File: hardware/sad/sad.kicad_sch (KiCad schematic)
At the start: 37 parts, among them IC1 LP5012RUKR, J1 USB_C_Receptacle_USB2.0_16P, U1 ATtiny1616-M, U2 MCP73831-2-OT

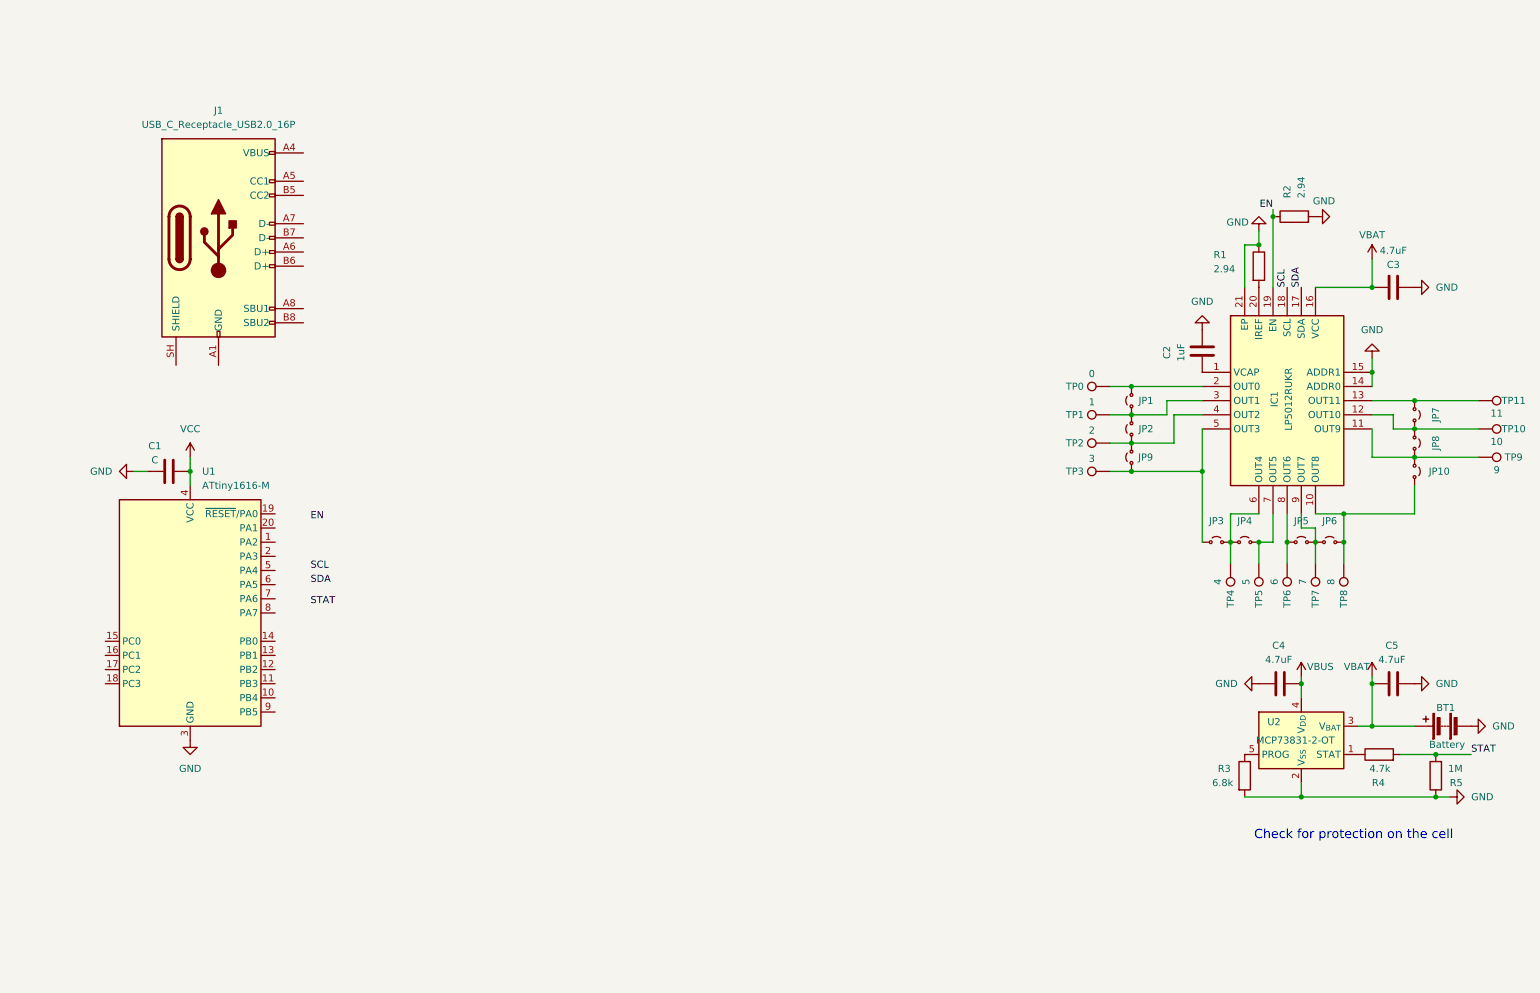
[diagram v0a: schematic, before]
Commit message: init sch finished
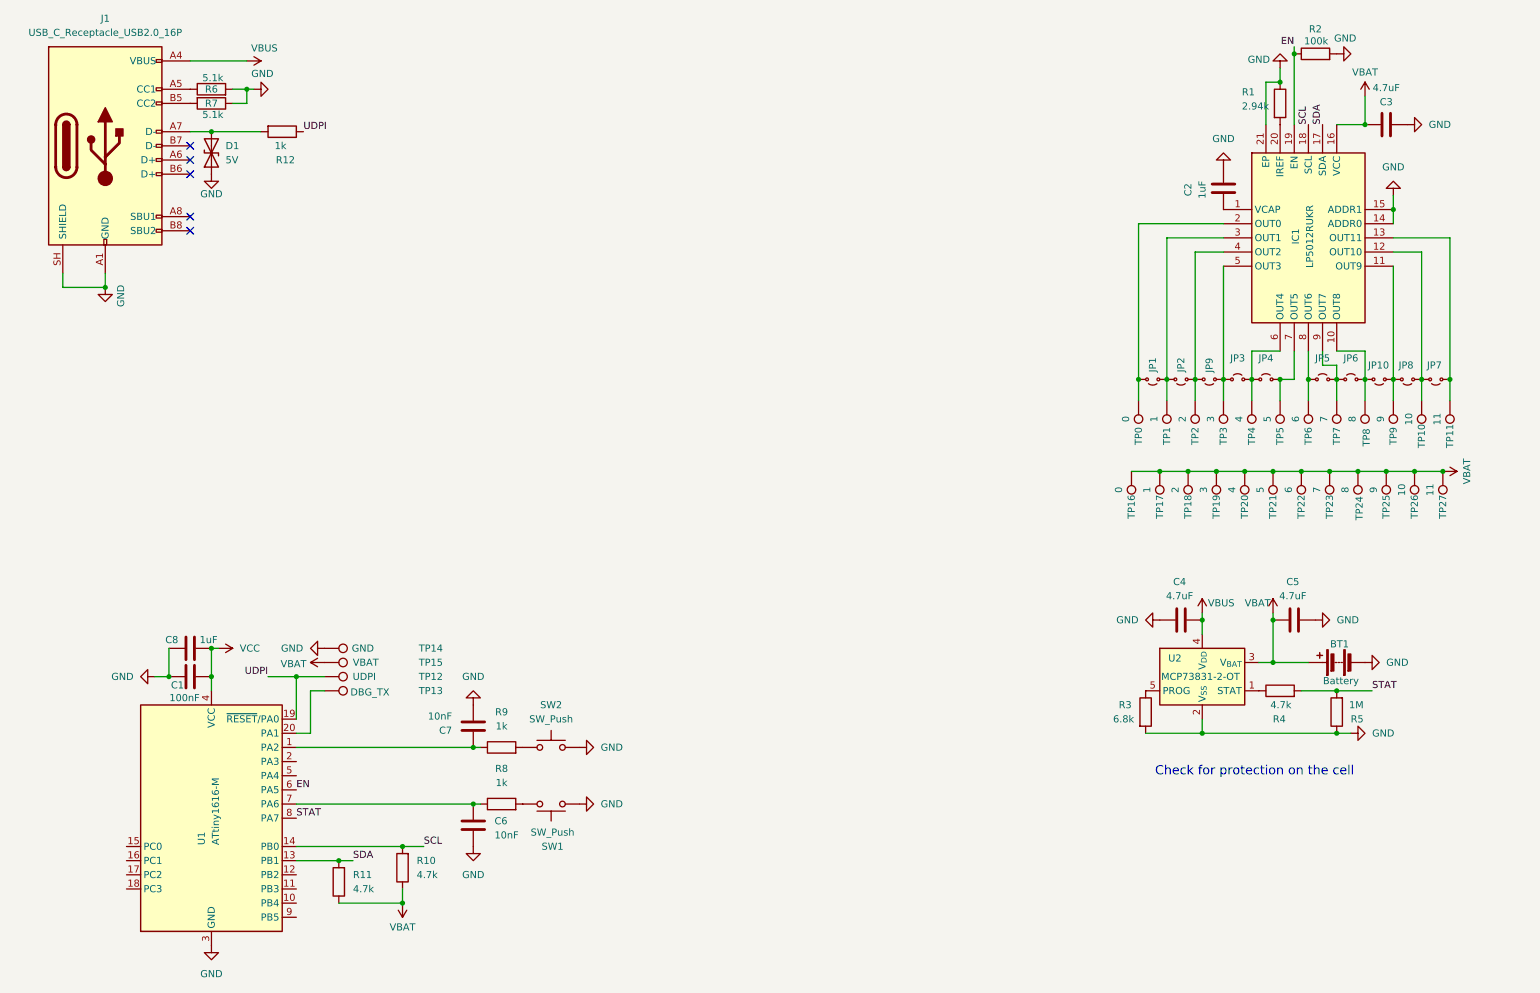
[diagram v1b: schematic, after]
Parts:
- added C6, C7: 10nF, Package_TO_SOT_SMD:SOT-23-5, symbol Device:C
- added C8: 1uF, Package_SO:SOIC-8_3.9x4.9mm_P1.27mm, symbol Device:C
- added D1: 5V, Package_DFN_QFN:QFN-16-1EP_4x4mm_P0.65mm_EP2.1x2.1mm_ThermalVias, symbol Device:D_TVS
- added R10, R11: 4.7k, Package_TO_SOT_SMD:SOT-23-5, symbol Device:R
- added R12, R8, R9: 1k, Package_TO_SOT_SMD:SOT-23-5, symbol Device:R
- added R6, R7: 5.1k, Package_TO_SOT_SMD:SOT-23-5, symbol Device:R
- added SW1, SW2: SW_Push, Button_Switch_SMD:Nidec_Copal_CAS-120A, symbol Switch:SW_Push
- added TP12: UDPI, Relay_THT:Relay_DPDT_Schrack-RT2-FormC_RM5mm, symbol Connector:TestPoint
- added TP13: DBG_TX, Relay_THT:Relay_DPDT_Schrack-RT2-FormC_RM5mm, symbol Connector:TestPoint
- added TP14: GND, Relay_THT:Relay_DPDT_Schrack-RT2-FormC_RM5mm, symbol Connector:TestPoint
- added TP15: VBAT, Relay_THT:Relay_DPDT_Schrack-RT2-FormC_RM5mm, symbol Connector:TestPoint
- added TP16: 0, Relay_THT:Relay_DPDT_Schrack-RT2-FormC_RM5mm, symbol Connector:TestPoint
- added TP17: 1, Relay_THT:Relay_DPDT_Schrack-RT2-FormC_RM5mm, symbol Connector:TestPoint
- added TP18: 2, Relay_THT:Relay_DPDT_Schrack-RT2-FormC_RM5mm, symbol Connector:TestPoint
- added TP19: 3, Relay_THT:Relay_DPDT_Schrack-RT2-FormC_RM5mm, symbol Connector:TestPoint
- added TP20: 4, Relay_THT:Relay_DPDT_Schrack-RT2-FormC_RM5mm, symbol Connector:TestPoint
- added TP21: 5, Relay_THT:Relay_DPDT_Schrack-RT2-FormC_RM5mm, symbol Connector:TestPoint
- added TP22: 6, Relay_THT:Relay_DPDT_Schrack-RT2-FormC_RM5mm, symbol Connector:TestPoint
- added TP23: 7, Relay_THT:Relay_DPDT_Schrack-RT2-FormC_RM5mm, symbol Connector:TestPoint
- added TP24: 8, Relay_THT:Relay_DPDT_Schrack-RT2-FormC_RM5mm, symbol Connector:TestPoint
- added TP25: 9, Relay_THT:Relay_DPDT_Schrack-RT2-FormC_RM5mm, symbol Connector:TestPoint
- added TP26: 10, Relay_THT:Relay_DPDT_Schrack-RT2-FormC_RM5mm, symbol Connector:TestPoint
- added TP27: 11, Relay_THT:Relay_DPDT_Schrack-RT2-FormC_RM5mm, symbol Connector:TestPoint
- C1: value C -> 100nF
- R1: value 2.94 -> 2.94k
- R2: value 2.94 -> 100k
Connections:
- net EN: now also U1.6 (PA5)
- net GND: now also J1.A1 (GND), J1.A12 (GND), J1.B1 (GND), J1.B12 (GND), J1.SH (SHIELD), C6.2, C7.2, C8.2, D1.1 (A1), R6.2, R7.1, SW1.1, SW2.2, TP14.1
- net SCL: now also U1.14 (PB0), R10.2
- net SDA: now also U1.13 (PB1), R11.2
- net STAT: now also U1.8 (PA7)
- net VBAT: now also R10.1, R11.1, TP15.1, TP16.1, TP17.1, TP18.1, TP19.1, TP20.1, TP21.1, TP22.1, TP23.1, TP24.1, TP25.1, TP26.1, TP27.1
- net VBUS: now also J1.A4 (VBUS), J1.A9 (VBUS), J1.B4 (VBUS), J1.B9 (VBUS)
- net VCC: now also C8.1
- net at U1.1 (PA2): now also C7.1, R9.1
- net UDPI: now reaches U1.19 (~{RESET}/PA0)
- net UDPI: now also R12.1, TP12.1
- net at U1.20 (PA1): now also TP13.1
- net at U1.7 (PA6): now also C6.1, R8.1
- net at J1.A5 (CC1): now also R6.1
- net at J1.A7 (D-): now also D1.2 (A2), R12.2
- net at J1.B5 (CC2): now also R7.2
- new net: R9.2, SW2.1
- new net: R8.2, SW1.2
- no-connect marks 0 -> 5
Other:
- moved on the sheet: BT1, C1, C2, C3, C4, C5, IC1, J1, JP1, JP10, JP2, JP3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

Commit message: rearranged
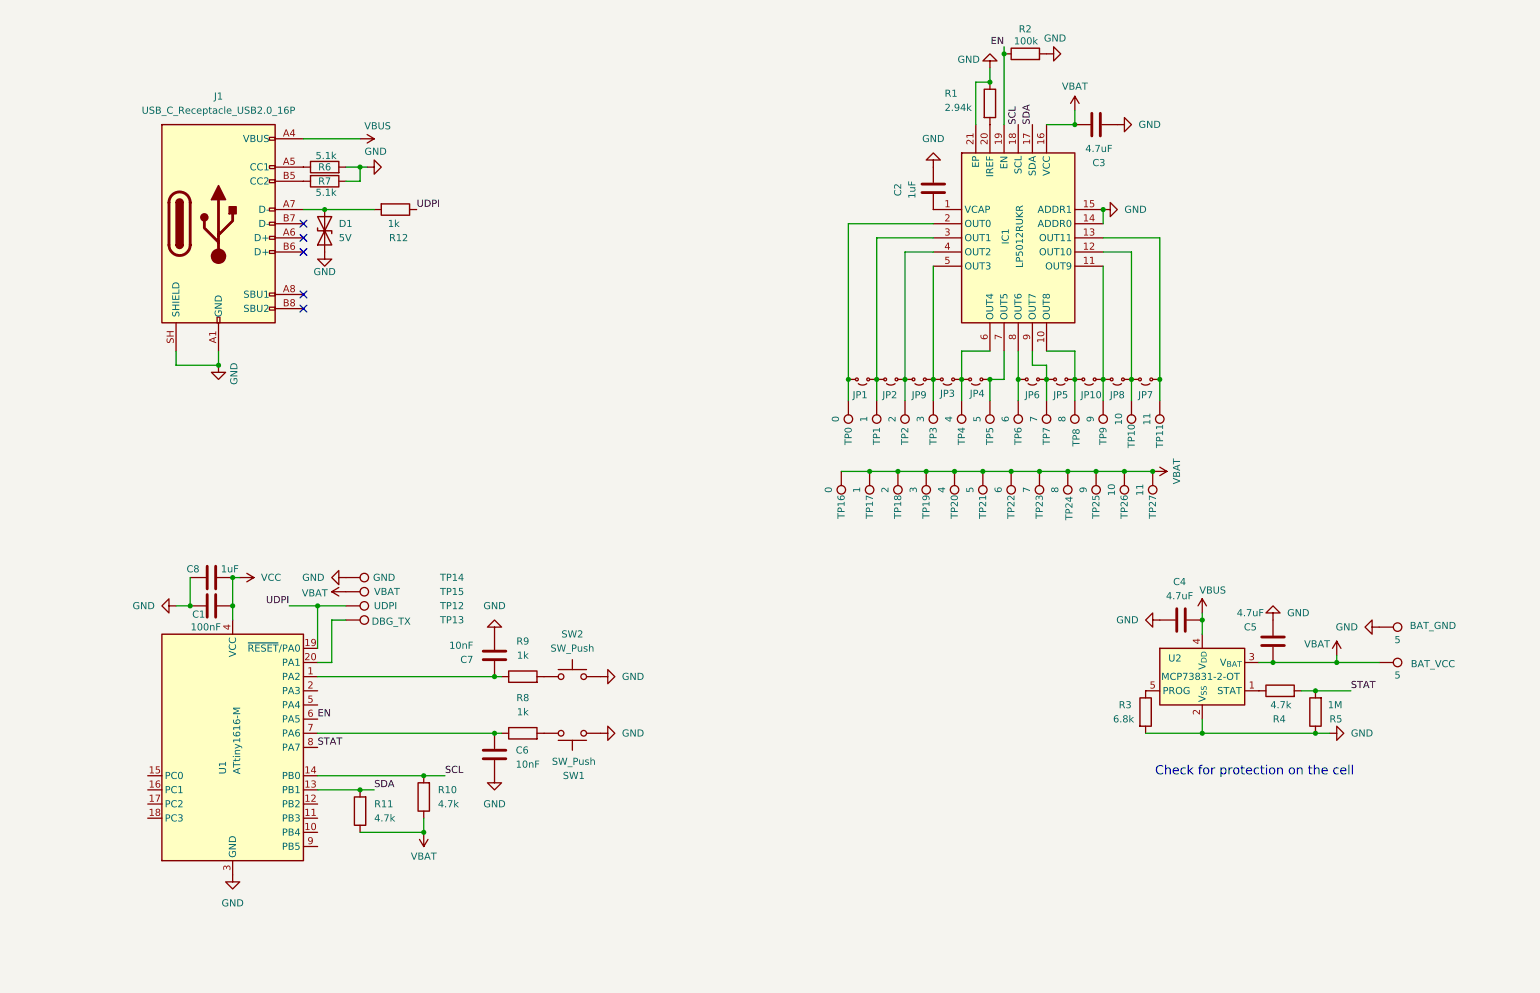
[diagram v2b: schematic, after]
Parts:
- removed BT1: Battery, Package_SON:Texas_DRC0010J_ThermalVias, symbol Device:Battery
- added BAT_GND, BAT_VCC: 5, Relay_THT:Relay_DPDT_Schrack-RT2-FormC_RM5mm, symbol Connector:TestPoint
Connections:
- net GND: now also BAT_GND.1
- net VBAT: now also BAT_VCC.1
- net at IC1.7 (OUT5), TP5.1: now also JP4.1 (A); no longer JP4.2 (B)
- net at IC1.8 (OUT6), TP6.1: now also JP6.2 (B); no longer JP5.1 (A)
- net at IC1.10 (OUT8), JP10.2 (B), TP8.1: now also JP5.1 (A); no longer JP6.2 (B)
- net at IC1.5 (OUT3), JP9.2 (B), TP3.1: now also JP3.2 (B); no longer JP3.1 (A)
- net at IC1.6 (OUT4), TP4.1: now also JP3.1 (A), JP4.2 (B); no longer JP3.2 (B), JP4.1 (A)
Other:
- moved on the sheet: C1, C2, C3, C5, C6, C7, C8, D1, IC1, J1, JP1, JP10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
